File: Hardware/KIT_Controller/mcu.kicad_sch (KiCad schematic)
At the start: 38 parts, among them J201 USB_B, J202 USB_BOOT, U201 TCA9554DB, U202 W25Q128JVS, U203 NCP1117-3.3_SOT223, U204 HDSP-7401, U205 RP2040, Y201 Crystal

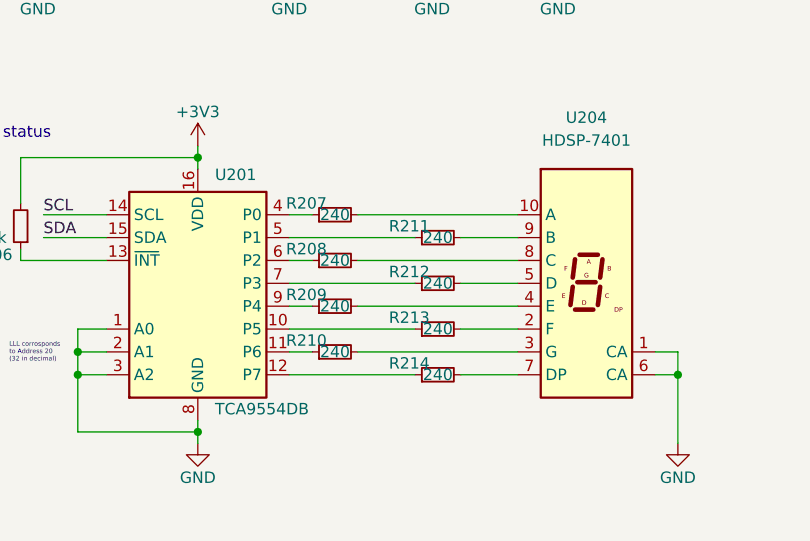
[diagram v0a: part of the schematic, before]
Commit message: Fixup drc
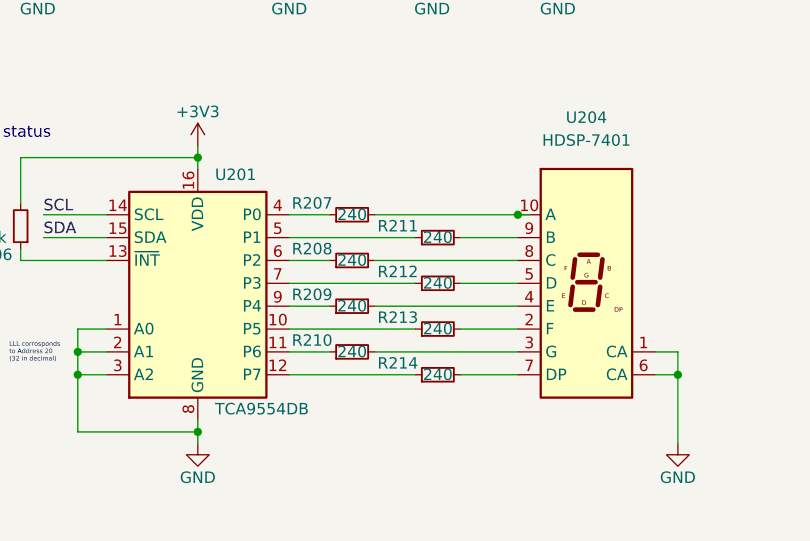
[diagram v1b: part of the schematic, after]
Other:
- moved on the sheet: R207, R208, R209, R210
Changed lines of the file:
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@@
   (junction (at 172.085 36.83) (diameter 0) (color 0 0 0 0)
+  )
+  (junction (at 73.025 163.195) (diameter 0) (color 0 0 0 0)
   )
   (junction (at 24.13 178.435) (diameter 0) (color 0 0 0 0)
@@
     (stroke (width 0) (type default) (color 0 0 0 0))
   )
-  (wire (pts (xy 47.625 173.355) (xy 50.165 173.355))
+  (wire (pts (xy 47.625 173.355) (xy 52.07 173.355))
     (stroke (width 0) (type default) (color 0 0 0 0))
   )
@@
     (stroke (width 0) (type default) (color 0 0 0 0))
   )
-  (wire (pts (xy 55.245 163.195) (xy 73.025 163.195))
+  (wire (pts (xy 57.15 163.195) (xy 73.025 163.195))
     (stroke (width 0) (type default) (color 0 0 0 0))
   )
@@
     (stroke (width 0) (type default) (color 0 0 0 0))
   )
+  (wire (pts (xy 74.295 163.195) (xy 73.025 163.195))
+    (stroke (width 0) (type default) (color 0 0 0 0))
+  )
   (wire (pts (xy 36.83 78.74) (xy 46.99 78.74))
     (stroke (width 0) (type default) (color 0 0 0 0))
@@
     (stroke (width 0) (type default) (color 0 0 0 0))
   )
-  (wire (pts (xy 55.245 178.435) (xy 73.025 178.435))
+  (wire (pts (xy 57.15 178.435) (xy 73.025 178.435))
     (stroke (width 0) (type default) (color 0 0 0 0))
   )
@@
     (stroke (width 0) (type default) (color 0 0 0 0))
   )
-  (wire (pts (xy 47.625 178.435) (xy 50.165 178.435))
+  (wire (pts (xy 47.625 178.435) (xy 52.07 178.435))
     (stroke (width 0) (type default) (color 0 0 0 0))
   )
@@
     (stroke (width 0) (type default) (color 0 0 0 0))
   )
-  (wire (pts (xy 55.245 173.355) (xy 73.025 173.355))
+  (wire (pts (xy 57.15 173.355) (xy 73.025 173.355))
     (stroke (width 0) (type default) (color 0 0 0 0))
   )
@@
     (stroke (width 0) (type default) (color 0 0 0 0))
   )
-  (wire (pts (xy 55.245 168.275) (xy 73.025 168.275))
+  (wire (pts (xy 57.15 168.275) (xy 73.025 168.275))
     (stroke (width 0) (type default) (color 0 0 0 0))
   )
@@
     (stroke (width 0) (type default) (color 0 0 0 0))
   )
-  (wire (pts (xy 47.625 163.195) (xy 50.165 163.195))
+  (wire (pts (xy 47.625 163.195) (xy 52.07 163.195))
     (stroke (width 0) (type default) (color 0 0 0 0))
   )
@@
     (stroke (width 0) (type default) (color 0 0 0 0))
   )
-  (wire (pts (xy 47.625 168.275) (xy 50.165 168.275))
+  (wire (pts (xy 47.625 168.275) (xy 52.07 168.275))
     (stroke (width 0) (type default) (color 0 0 0 0))
   )
@@
     (pin "2")
   )
-  (symbol (lib_id "Device:R_Small") (at 52.705 173.355 90) (unit 1)
-    (in_bom yes) (on_board yes)
-    (property "Reference" "R209" (id 0) (at 49.53 172.085 90))
-    (property "Value" "240" (id 1) (at 52.705 173.355 90))
-    (property "Footprint" "Resistor_SMD:R_0805_2012Metric" (id 2) (at 52.705 173.355 0)
-      (effects (font (size 1.27 1.27)) hide)
-    )
-    (property "Datasheet" "~" (id 3) (at 52.705 173.355 0)
+  (symbol (lib_id "Device:R_Small") (at 54.61 173.355 90) (unit 1)
+    (in_bom yes) (on_board yes)
+    (property "Reference" "R209" (id 0) (at 50.165 172.085 90))
+    (property "Value" "240" (id 1) (at 54.61 173.355 90))
+    (property "Footprint" "Resistor_SMD:R_0805_2012Metric" (id 2) (at 54.61 173.355 0)
+      (effects (font (size 1.27 1.27)) hide)
+    )
+    (property "Datasheet" "~" (id 3) (at 54.61 173.355 0)
       (effects (font (size 1.27 1.27)) hide)
     )
@@
   (symbol (lib_id "Device:R_Small") (at 64.135 175.895 90) (unit 1)
     (in_bom yes) (on_board yes)
-    (property "Reference" "R213" (id 0) (at 60.96 174.625 90))
+    (property "Reference" "R213" (id 0) (at 59.69 174.625 90))
     (property "Value" "240" (id 1) (at 64.135 175.895 90))
     (property "Footprint" "Resistor_SMD:R_0805_2012Metric" (id 2) (at 64.135 175.895 0)
@@
     (pin "2")
   )
-  (symbol (lib_id "Device:R_Small") (at 52.705 163.195 90) (unit 1)
-    (in_bom yes) (on_board yes)
-    (property "Reference" "R207" (id 0) (at 49.53 161.925 90))
-    (property "Value" "240" (id 1) (at 52.705 163.195 90))
-    (property "Footprint" "Resistor_SMD:R_0805_2012Metric" (id 2) (at 52.705 163.195 0)
-      (effects (font (size 1.27 1.27)) hide)
-    )
-    (property "Datasheet" "~" (id 3) (at 52.705 163.195 0)
+  (symbol (lib_id "Device:R_Small") (at 54.61 163.195 90) (unit 1)
+    (in_bom yes) (on_board yes)
+    (property "Reference" "R207" (id 0) (at 50.165 161.925 90))
+    (property "Value" "240" (id 1) (at 54.61 163.195 90))
+    (property "Footprint" "Resistor_SMD:R_0805_2012Metric" (id 2) (at 54.61 163.195 0)
+      (effects (font (size 1.27 1.27)) hide)
+    )
+    (property "Datasheet" "~" (id 3) (at 54.61 163.195 0)
       (effects (font (size 1.27 1.27)) hide)
     )
@@
   (symbol (lib_id "Device:R_Small") (at 64.135 165.735 90) (unit 1)
     (in_bom yes) (on_board yes)
-    (property "Reference" "R211" (id 0) (at 60.96 164.465 90))
+    (property "Reference" "R211" (id 0) (at 59.69 164.465 90))
     (property "Value" "240" (id 1) (at 64.135 165.735 90))
     (property "Footprint" "Resistor_SMD:R_0805_2012Metric" (id 2) (at 64.135 165.735 0)
@@
     (pin "3")
   )
-  (symbol (lib_id "Device:R_Small") (at 52.705 178.435 90) (unit 1)
-    (in_bom yes) (on_board yes)
-    (property "Reference" "R210" (id 0) (at 49.53 177.165 90))
-    (property "Value" "240" (id 1) (at 52.705 178.435 90))
-    (property "Footprint" "Resistor_SMD:R_0805_2012Metric" (id 2) (at 52.705 178.435 0)
-      (effects (font (size 1.27 1.27)) hide)
-    )
-    (property "Datasheet" "~" (id 3) (at 52.705 178.435 0)
+  (symbol (lib_id "Device:R_Small") (at 54.61 178.435 90) (unit 1)
+    (in_bom yes) (on_board yes)
+    (property "Reference" "R210" (id 0) (at 50.165 177.165 90))
+    (property "Value" "240" (id 1) (at 54.61 178.435 90))
+    (property "Footprint" "Resistor_SMD:R_0805_2012Metric" (id 2) (at 54.61 178.435 0)
+      (effects (font (size 1.27 1.27)) hide)
+    )
+    (property "Datasheet" "~" (id 3) (at 54.61 178.435 0)
       (effects (font (size 1.27 1.27)) hide)
     )
@@
   (symbol (lib_id "Device:R_Small") (at 64.135 170.815 90) (unit 1)
     (in_bom yes) (on_board yes)
-    (property "Reference" "R212" (id 0) (at 60.96 169.545 90))
+    (property "Reference" "R212" (id 0) (at 59.69 169.545 90))
     (property "Value" "240" (id 1) (at 64.135 170.815 90))
     (property "Footprint" "Resistor_SMD:R_0805_2012Metric" (id 2) (at 64.135 170.815 0)
@@
   (symbol (lib_id "Device:R_Small") (at 64.135 180.975 90) (unit 1)
     (in_bom yes) (on_board yes)
-    (property "Reference" "R214" (id 0) (at 60.96 179.705 90))
+    (property "Reference" "R214" (id 0) (at 59.69 179.705 90))
     (property "Value" "240" (id 1) (at 64.135 180.975 90))
     (property "Footprint" "Resistor_SMD:R_0805_2012Metric" (id 2) (at 64.135 180.975 0)
@@
     (pin "1")
   )
-  (symbol (lib_id "Device:R_Small") (at 52.705 168.275 90) (unit 1)
-    (in_bom yes) (on_board yes)
-    (property "Reference" "R208" (id 0) (at 49.53 167.005 90))
-    (property "Value" "240" (id 1) (at 52.705 168.275 90))
-    (property "Footprint" "Resistor_SMD:R_0805_2012Metric" (id 2) (at 52.705 168.275 0)
-      (effects (font (size 1.27 1.27)) hide)
-    )
-    (property "Datasheet" "~" (id 3) (at 52.705 168.275 0)
-      (effects (font (size 1.27 1.27)) hide)
-    )
+  (symbol (lib_id "Device:R_Small") (at 54.61 168.275 90) (unit 1)
+    (in_bom yes) (on_board yes)
+    (property "Reference" "R208" (id 0) (at 50.165 167.005 90))
+    (property "Value" "240" (id 1) (at 54.61 168.275 90))
+    (property "Footprint" "Resistor_SMD:R_0805_2012Metric" (id 2) (at 54.61 168.275 0)
+      (effects (font (size 1.27 1.27)) hide)
+    )
+    (property "Datasheet" "~" (id 3) (at 54.61 168.275 0)
+      (effects (font (size 1.27 1.27)) hide)
+    )
